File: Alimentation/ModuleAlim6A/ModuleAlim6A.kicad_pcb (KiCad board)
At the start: 2 copper layers, 40 x 52 mm, 12 parts, among them J1 Inhibit, J2 Alim. IN / OUT, U1 PTN78020W_EUK-7

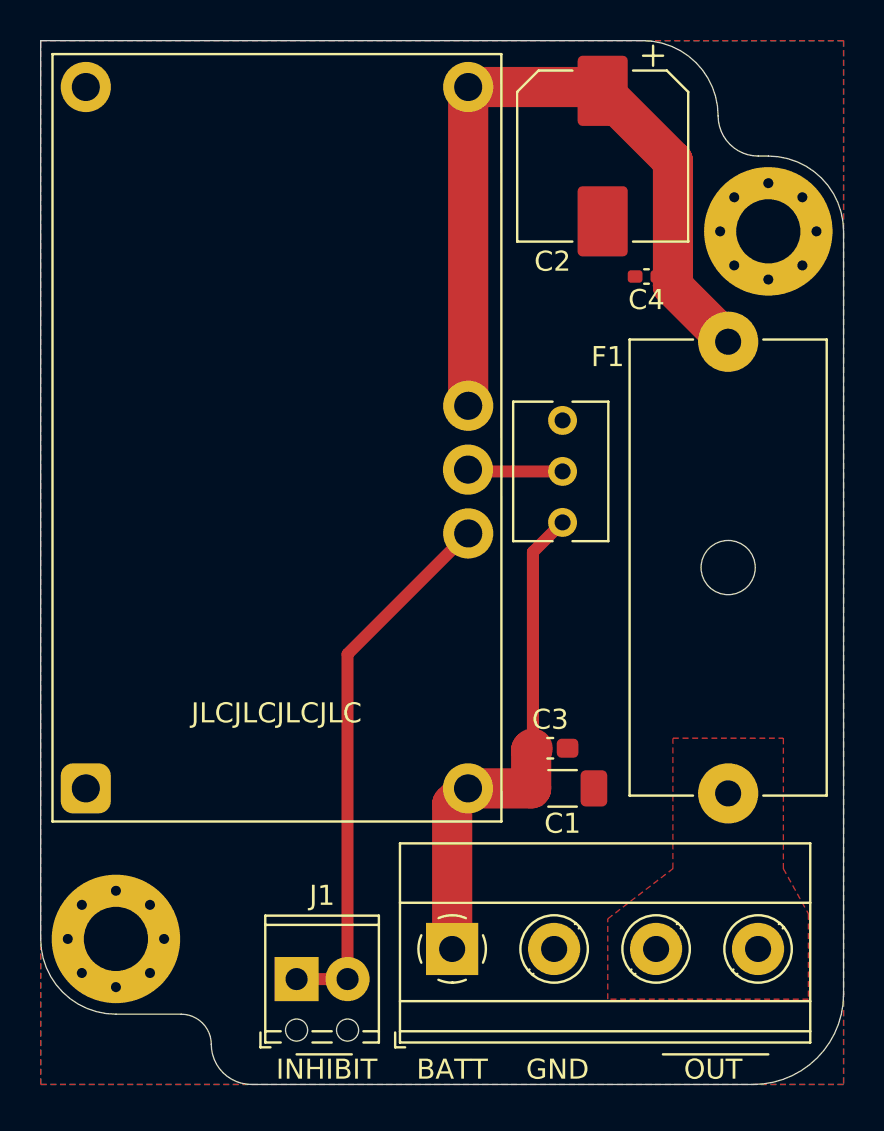
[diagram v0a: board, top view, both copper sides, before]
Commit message: Finalisation alimentations
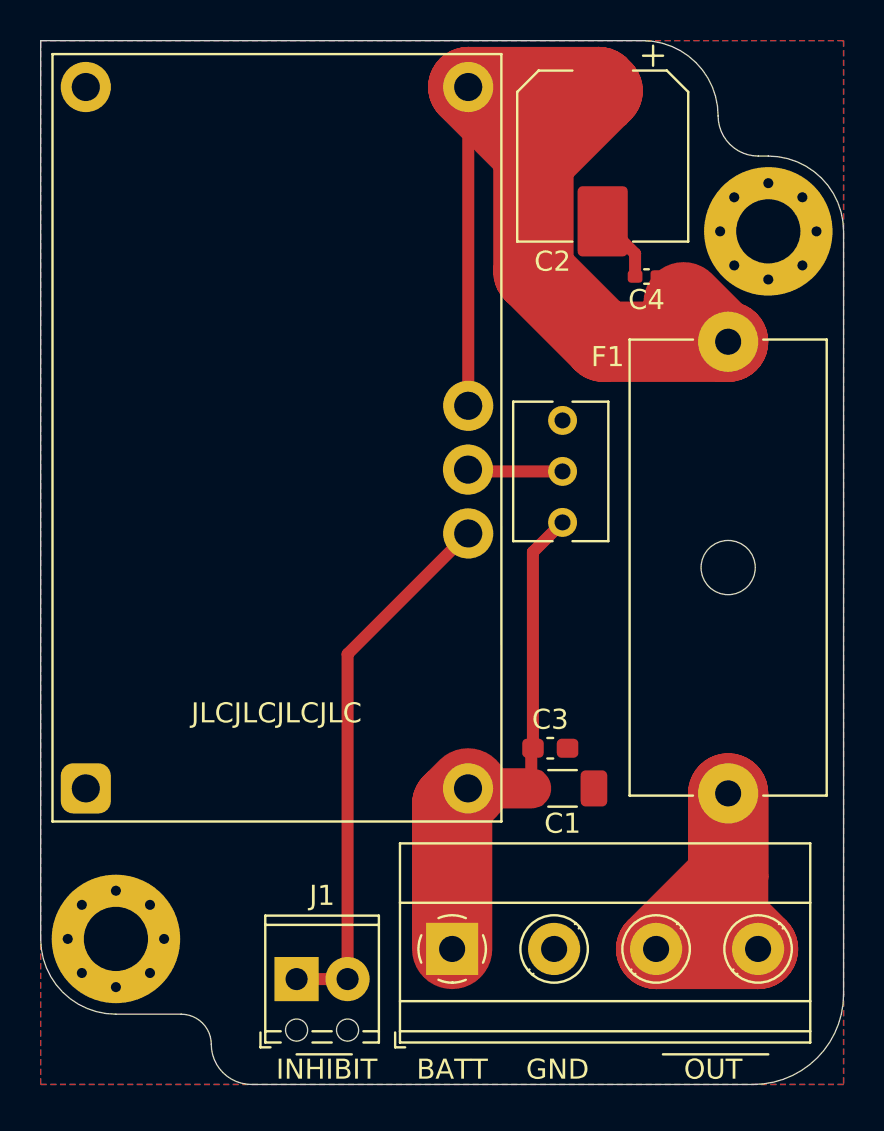
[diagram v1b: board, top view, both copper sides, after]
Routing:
- net /OUT: track 0.00 -> 22.7 mm
- net Net-(C2-Pad1): track 37.7 -> 52.3 mm
- net GND: track 0.00 -> 3.42 mm
- removed copper zone on F.Cu, net /OUT
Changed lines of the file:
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@@
     (thickness 1.6)
     (drawings 26)
-    (tracks 19)
+    (tracks 31)
     (zones 0)
     (modules 12)
@@
   )
   (setup
-    (last_trace_width 0.25)
+    (last_trace_width 4)
     (user_trace_width 0.6)
     (user_trace_width 2)
+    (user_trace_width 4)
     (trace_clearance 0.2)
     (zone_clearance 0.508)
@@
   (gr_line (start 165.25 91) (end 165.25 129) (layer Edge.Cuts) (width 0.05))
   (gr_line (start 125.25 81.5) (end 155.25 81.5) (layer Edge.Cuts) (width 0.05))
-  (segment (start 145.75 119.54) (end 146.54 118.75) (width 2) (layer F.Cu) (net 2))
-  (segment (start 145.75 126.75) (end 145.75 119.54) (width 2) (layer F.Cu) (net 2))
-  (segment (start 146.54 118.75) (end 149.6875 118.75) (width 2) (layer F.Cu) (net 2))
-  (segment (start 149.6875 116.8375) (end 149.76249 116.76251) (width 2) (layer F.Cu) (net 2))
-  (segment (start 149.6875 118.75) (end 149.6875 116.8375) (width 2) (layer F.Cu) (net 2))
+  (segment (start 154.865 92.115) (end 153.25 90.5) (width 0.6) (layer F.Cu) (net 1))
+  (segment (start 154.865 93.25) (end 154.865 92.115) (width 0.6) (layer F.Cu) (net 1))
   (segment (start 149.775 106.975) (end 151.25 105.5) (width 0.6) (layer F.Cu) (net 2))
   (segment (start 149.775 116.75) (end 149.775 106.975) (width 0.6) (layer F.Cu) (net 2))
+  (segment (start 145.75 119.54) (end 146.54 118.75) (width 4) (layer F.Cu) (net 2))
+  (segment (start 145.75 126.75) (end 145.75 119.54) (width 4) (layer F.Cu) (net 2))
+  (segment (start 146.54 118.75) (end 149.6875 118.75) (width 2) (layer F.Cu) (net 2))
+  (segment (start 149.6875 116.8375) (end 149.775 116.75) (width 0.6) (layer F.Cu) (net 2))
+  (segment (start 149.6875 118.75) (end 149.6875 116.8375) (width 0.6) (layer F.Cu) (net 2))
+  (segment (start 159.5 125.26) (end 160.99 126.75) (width 4) (layer F.Cu) (net 3))
+  (segment (start 159.5 119) (end 159.5 125.26) (width 4) (layer F.Cu) (net 3))
+  (segment (start 159.5 123.16) (end 155.91 126.75) (width 4) (layer F.Cu) (net 3))
+  (segment (start 159.5 119) (end 159.5 123.16) (width 4) (layer F.Cu) (net 3))
+  (segment (start 155.91 126.75) (end 160.99 126.75) (width 4) (layer F.Cu) (net 3))
   (segment (start 138 128.25) (end 140.54 128.25) (width 0.6) (layer F.Cu) (net 4))
   (segment (start 140.5 128.21) (end 140.54 128.25) (width 0.6) (layer F.Cu) (net 4))
@@
   (segment (start 146.63 102.96) (end 146.54 102.87) (width 0.6) (layer F.Cu) (net 5))
   (segment (start 151.25 102.96) (end 146.63 102.96) (width 0.6) (layer F.Cu) (net 5))
-  (segment (start 146.55 99.69) (end 146.55 83.81) (width 2) (layer F.Cu) (net 6))
-  (segment (start 153.06 83.81) (end 153.25 84) (width 2) (layer F.Cu) (net 6))
-  (segment (start 146.55 83.81) (end 153.06 83.81) (width 2) (layer F.Cu) (net 6))
-  (segment (start 159.5 96.5) (end 156.75 93.75) (width 2) (layer F.Cu) (net 6))
-  (segment (start 156.75 87.5) (end 153.25 84) (width 2) (layer F.Cu) (net 6))
-  (segment (start 156.75 93.75) (end 156.75 87.5) (width 2) (layer F.Cu) (net 6))
+  (segment (start 146.55 99.69) (end 146.55 83.81) (width 0.6) (layer F.Cu) (net 6))
+  (segment (start 153.06 83.81) (end 153.25 84) (width 4) (layer F.Cu) (net 6))
+  (segment (start 146.55 83.81) (end 153.06 83.81) (width 4) (layer F.Cu) (net 6))
+  (segment (start 159.25 96.5) (end 157.281495 94.531495) (width 4) (layer F.Cu) (net 6))
+  (segment (start 159.5 96.5) (end 159.25 96.5) (width 4) (layer F.Cu) (net 6))
+  (segment (start 153.28516 96.5) (end 159.5 96.5) (width 4) (layer F.Cu) (net 6))
+  (segment (start 149.79999 93.01483) (end 153.28516 96.5) (width 4) (layer F.Cu) (net 6))
+  (segment (start 149.79999 87.45001) (end 149.79999 93.01483) (width 4) (layer F.Cu) (net 6))
+  (segment (start 153.25 84) (end 149.79999 87.45001) (width 4) (layer F.Cu) (net 6))
+  (segment (start 149.79999 87.05999) (end 149.79999 87.45001) (width 4) (layer F.Cu) (net 6))
+  (segment (start 146.55 83.81) (end 149.79999 87.05999) (width 4) (layer F.Cu) (net 6))
   (zone (net 1) (net_name GND) (layer B.Cu) (hatch edge 0.508)
     (connect_pads (clearance 0.508))
@@
       )
     )
-  )
-  (zone (net 3) (net_name /OUT) (layer F.Cu) (hatch edge 0.508)
-    (priority 1)
-    (connect_pads (clearance 0.508))
-    (min_thickness 0.508)
-    (fill yes (arc_segments 32) (thermal_gap 0.508) (thermal_bridge_width 1.016) (smoothing fillet) (radius 2))
-    (polygon
-      (pts
-        (xy 162.25 122.75) (xy 163.5 125) (xy 163.5 129.25) (xy 153.5 129.25) (xy 153.5 125.25)
-        (xy 156.75 122.75) (xy 156.75 116.25) (xy 162.25 116.25)
-      )
-    )

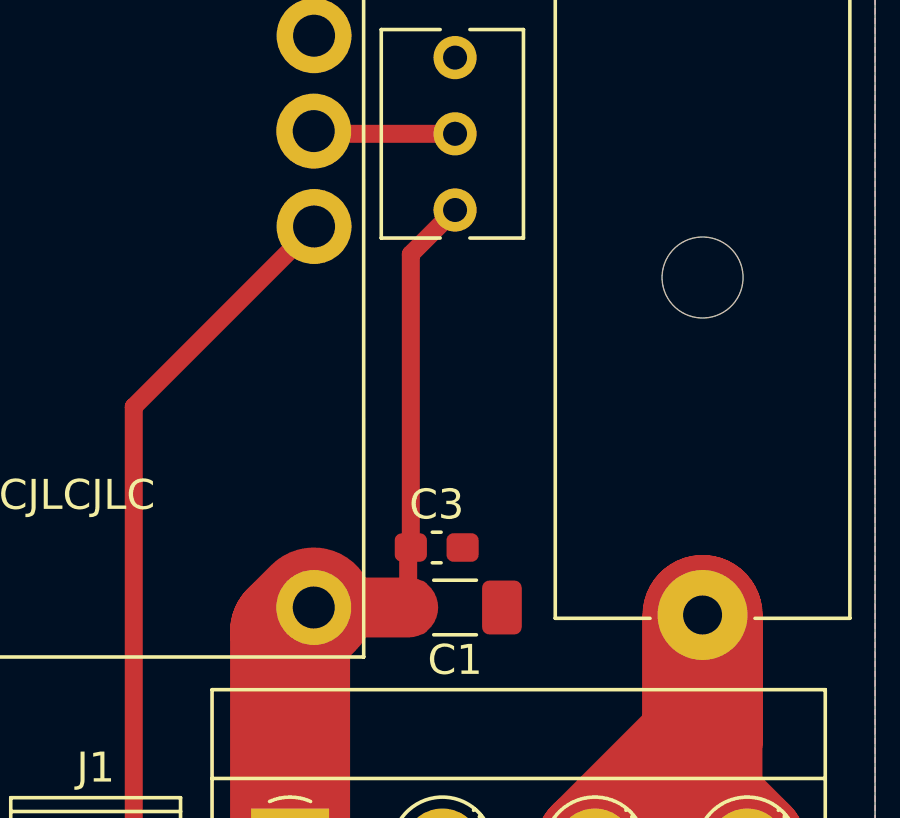
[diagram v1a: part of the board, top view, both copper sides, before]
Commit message: Finalisation pour commande pack Alimentation 14/02/2021
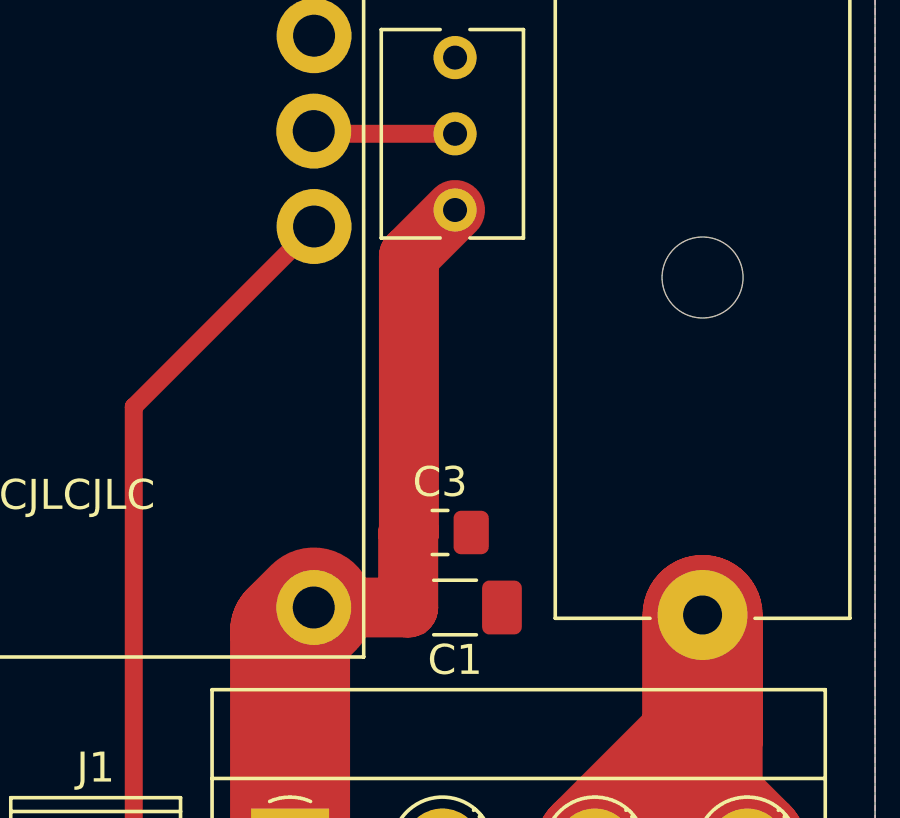
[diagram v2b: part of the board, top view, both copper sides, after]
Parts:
- C3: footprint Capacitor_SMD:C_0603_1608Metric_Pad1.08x0.95mm_HandSolder -> Capacitor_SMD:C_0805_2012Metric_Pad1.18x1.45mm_HandSolder
- moved C3 0.51 mm to (150.8, 116.2)
